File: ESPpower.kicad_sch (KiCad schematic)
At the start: 58 parts, among them CON1 +7 TO +20VDC, J1 RJ12, J2 Display, J3 Conn_01x02_Male, J4 Conn_01x02_Male, M1 ESP-12, P1 Program, Q1 AO3400, SW1 Reset, SW2 Program, U1 AP1117-3.3, U13 DS3231M, U2 PCF8574, U3 MP2363, U4 FM24C256, U5 74125, U6 MAX485

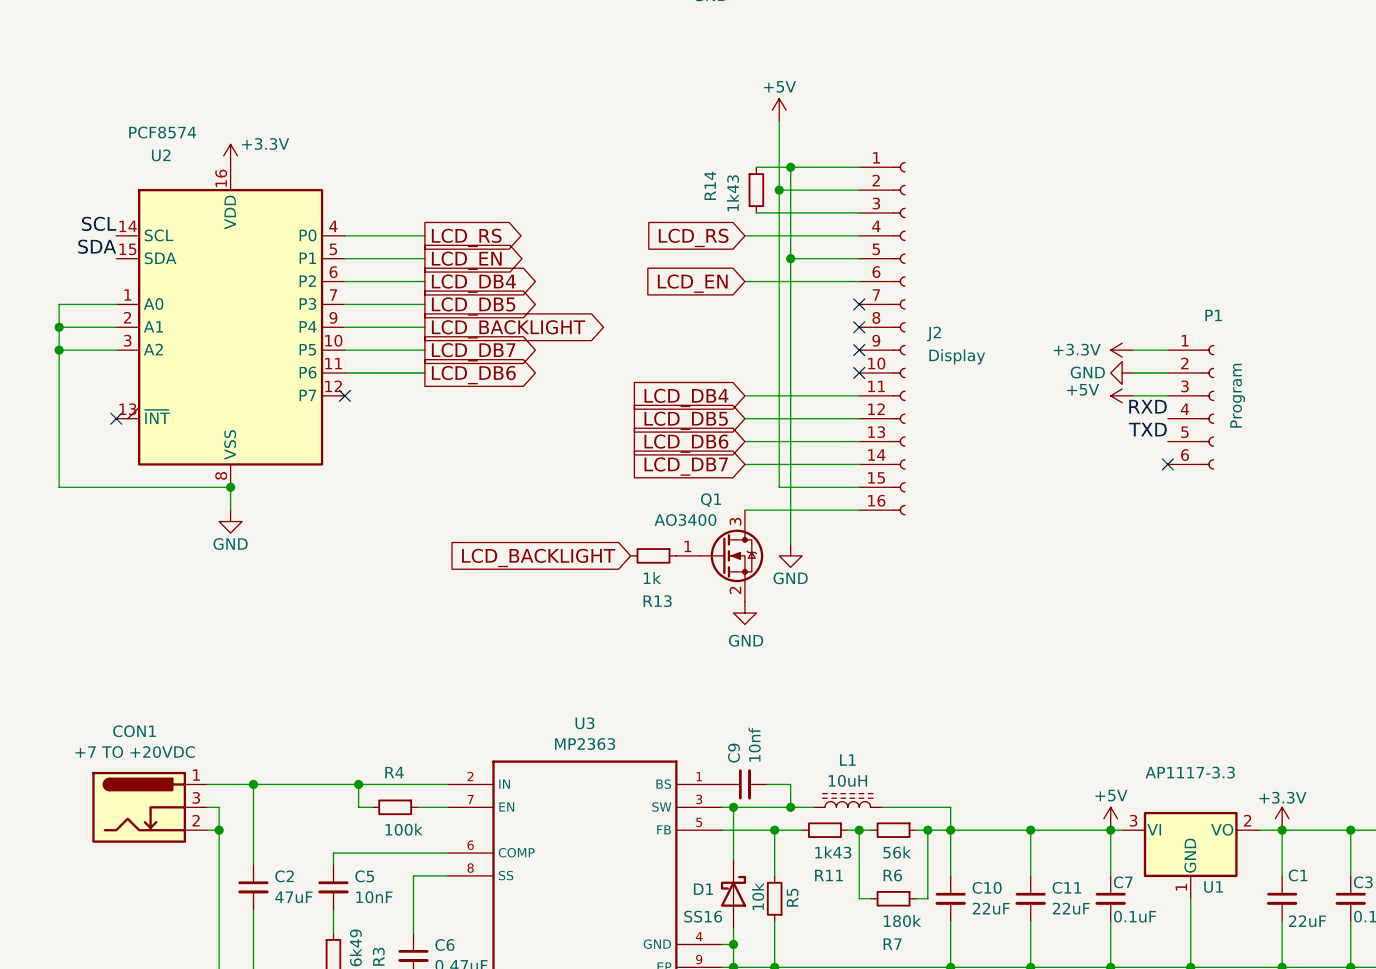
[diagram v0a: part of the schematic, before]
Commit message: Saved with later KiCAD version.
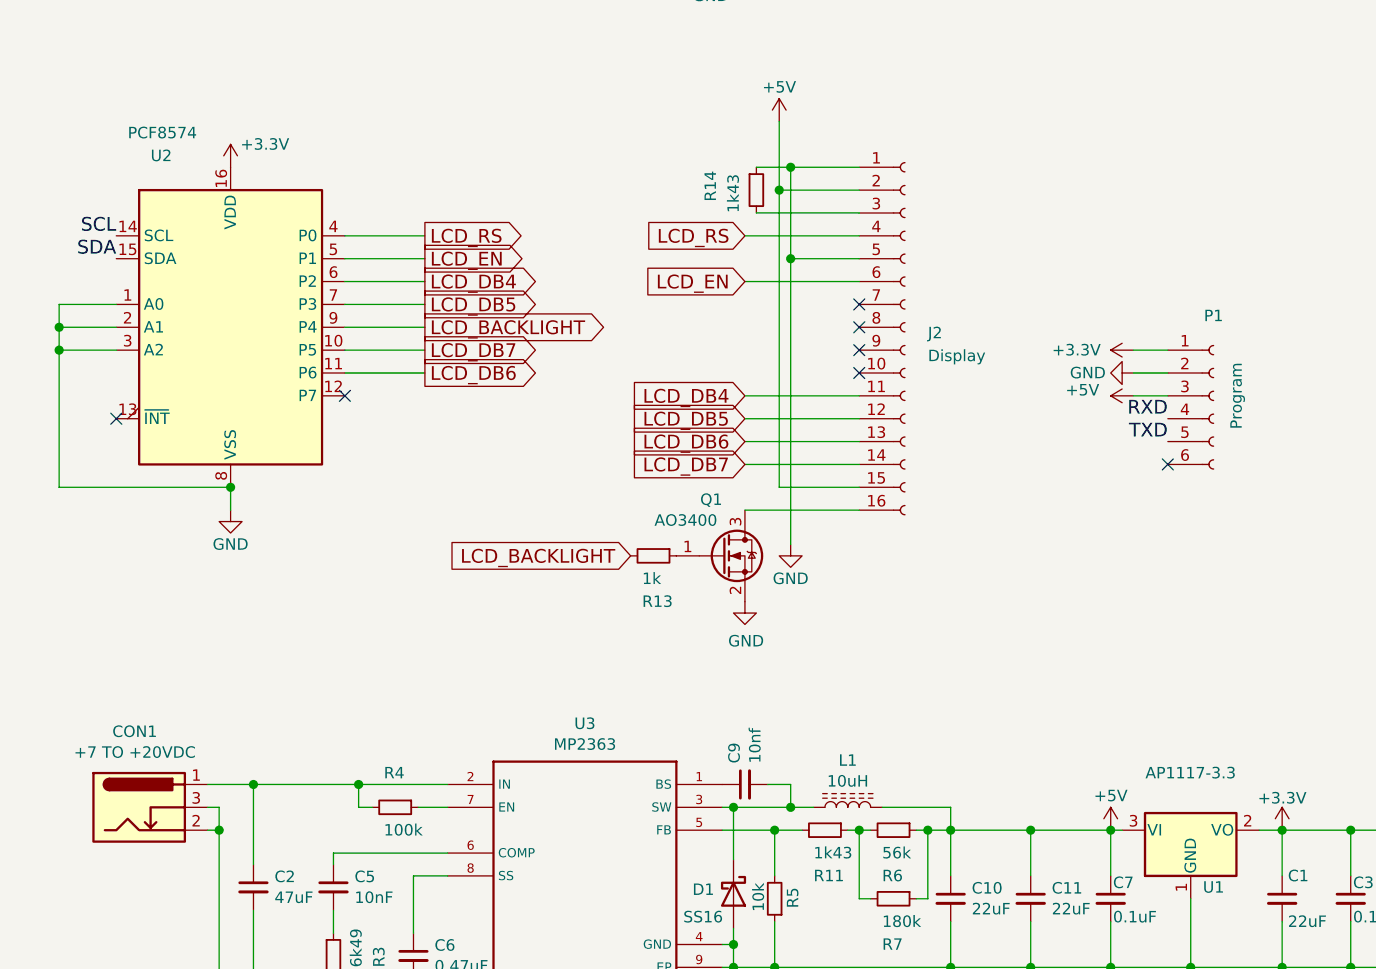
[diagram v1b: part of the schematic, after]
